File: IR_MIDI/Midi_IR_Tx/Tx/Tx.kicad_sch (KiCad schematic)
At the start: 16 parts, among them J1 MIDI in, J2 MIDI Thr, Q1 2N3904, Q2 2N3904, Q3 2N3904, Q4 2N3904, Y1 1MHz

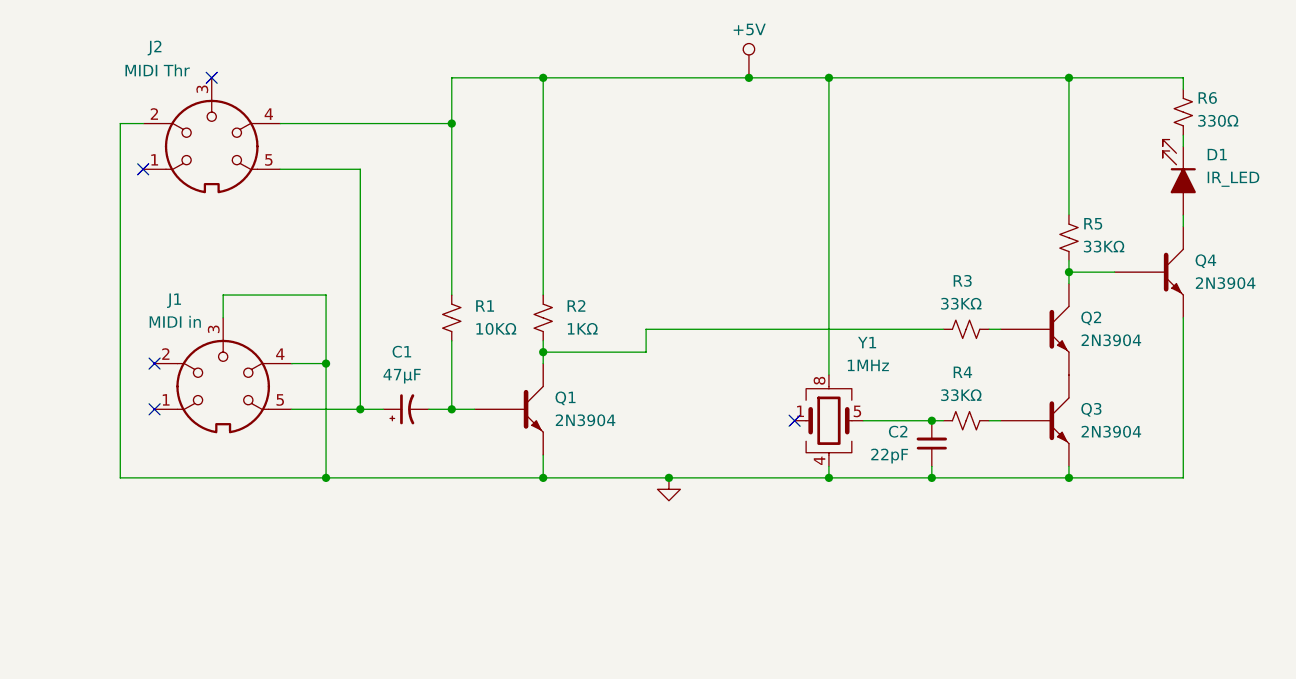
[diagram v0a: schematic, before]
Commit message: updating for merge
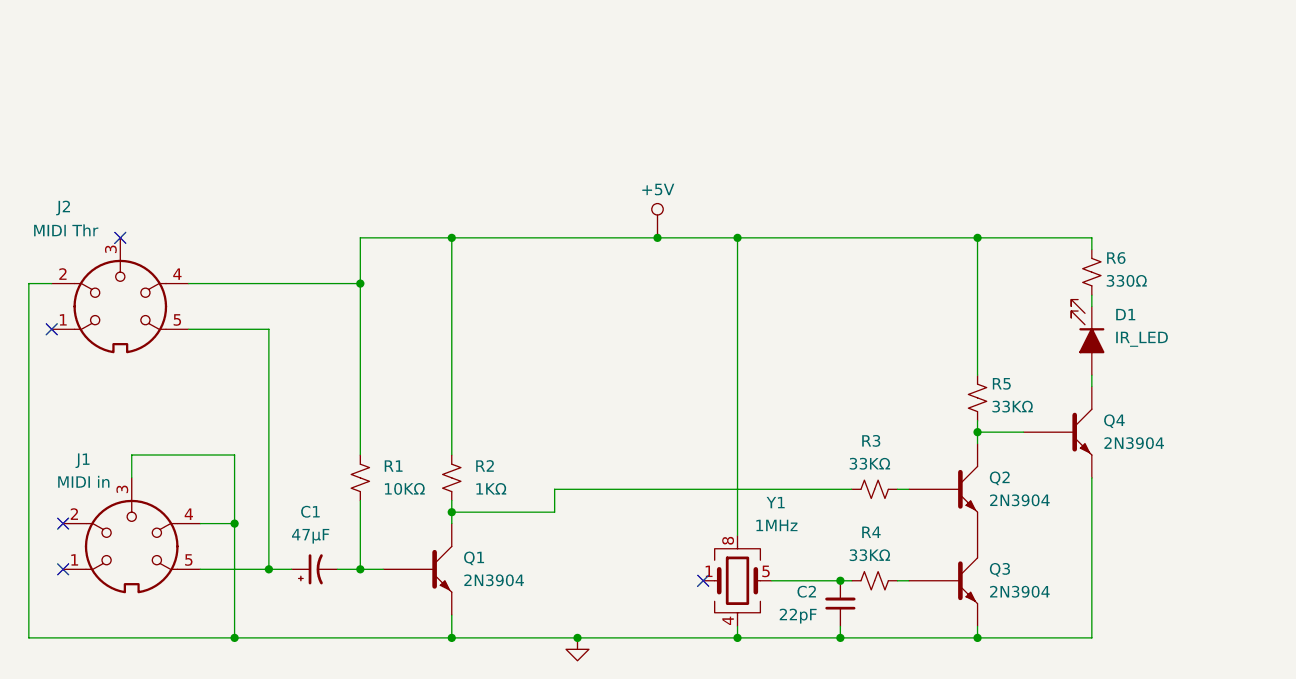
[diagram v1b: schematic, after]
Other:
- moved on the sheet: C1, C2, D1, J1, J2, Q1, Q2, Q3, Q4, R1, R2, R3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
